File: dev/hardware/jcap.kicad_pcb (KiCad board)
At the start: 2 copper layers, 140 x 87 mm, 74 parts, among them J201 CPU PGMR, J202 GPU PGMR, J203 SPARE GPU HDR, J204 SPARE CPU HDR, J301 DC IN, J502 VGA OUT, J601 CONTROLS, SW201 CPU ~{RES}, SW202 GPU ~{RES}, SW203 DEBUG, SW601 TILT, U101 P8X32A-D40, U201 P8X32A-D40, U302 LF33_TO220, U401 24LC256, U402 24LC256, U601 74HC165, U602 74HC165, Y101 6.5MHz, Y201 6.5MHz

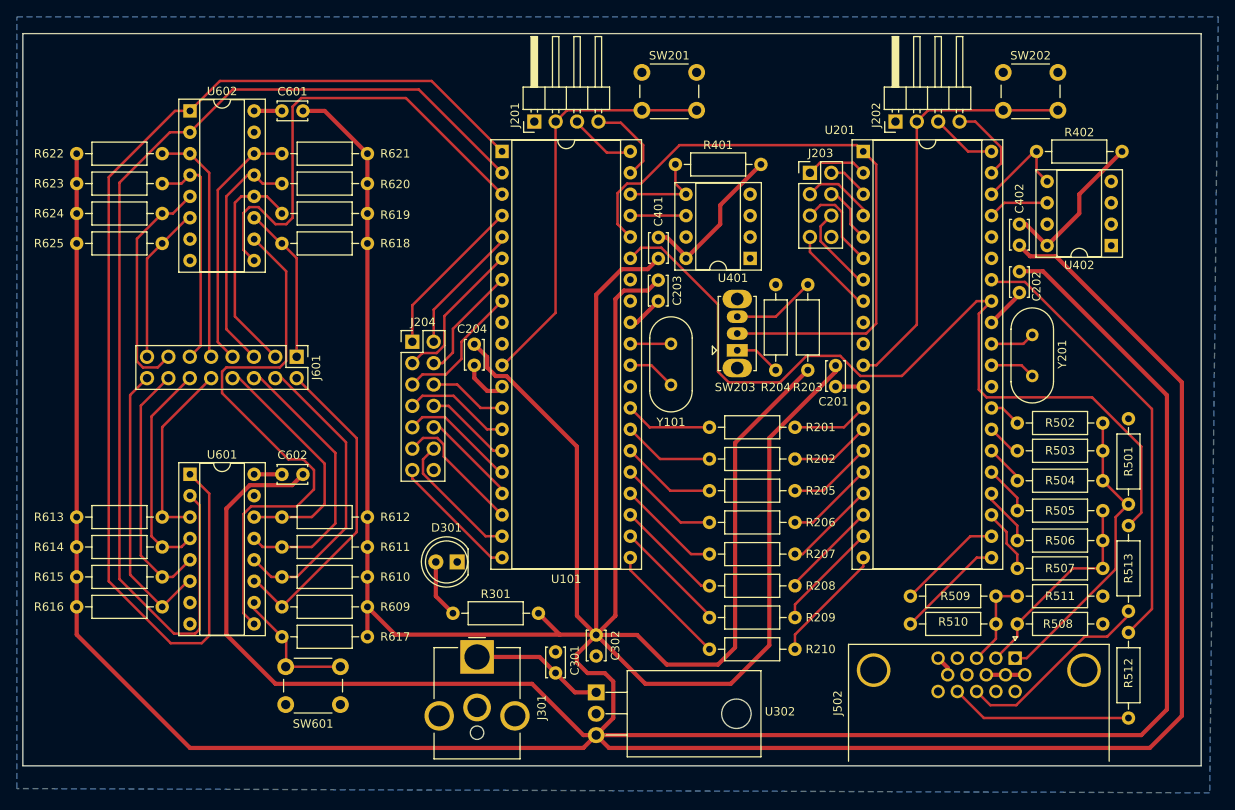
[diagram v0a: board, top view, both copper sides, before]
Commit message: Finalized optimized board layout
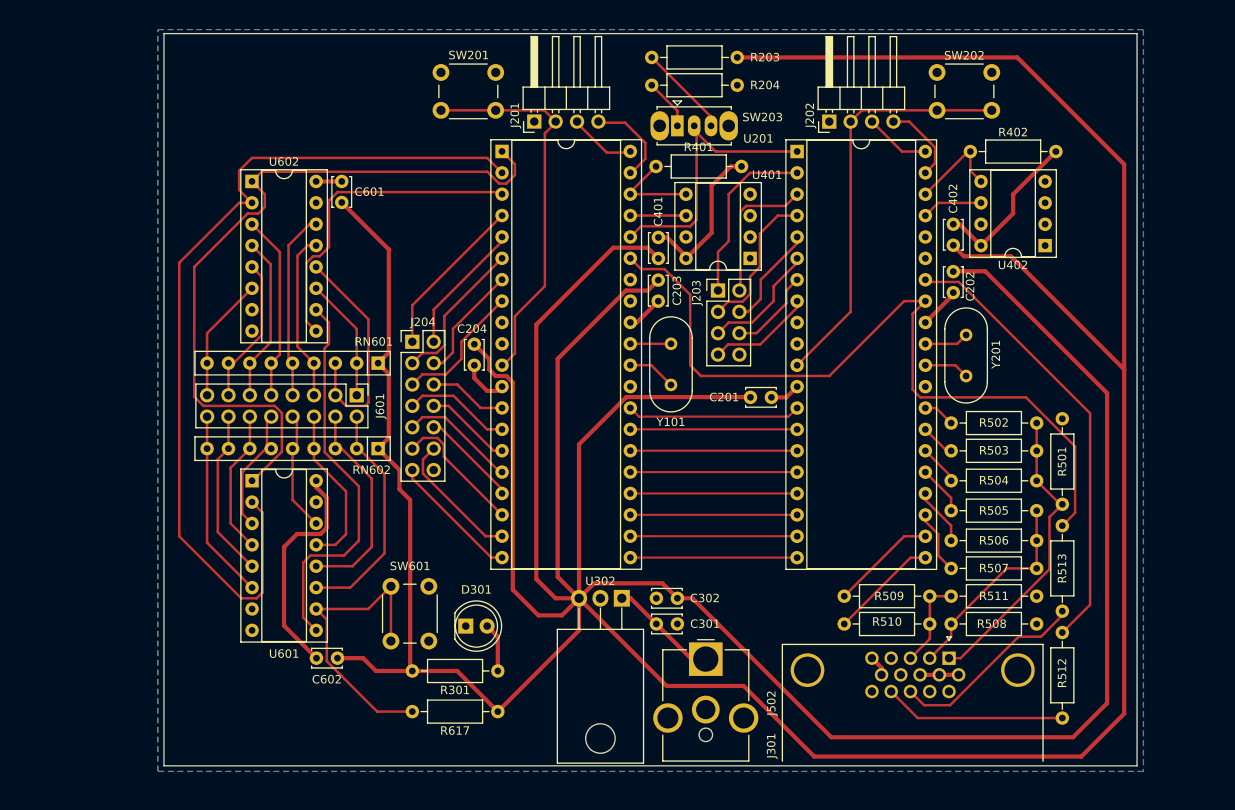
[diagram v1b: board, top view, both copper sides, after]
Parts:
- removed R201, R202, R205, R206, R207, R208, R209, R210: 200, Resistor_THT:R_Axial_DIN0207_L6.3mm_D2.5mm_P10.16mm_Horizontal
- removed R609, R610, R611, R612, R613, R614, R615, R616, R618, R619, R620, R621, R622, R623, R624, R625: 10K, Resistor_THT:R_Axial_DIN0207_L6.3mm_D2.5mm_P10.16mm_Horizontal
- added RN601: 10K, Resistor_THT:R_Array_SIP9, F.Cu at (124.2, 105.2)
- added RN602: 10K, Resistor_THT:R_Array_SIP9, F.Cu at (124.2, 115.3)
- moved R203 32.8 mm to (156.7, 68.8), turned to 0 degrees
- moved SW203 27.6 mm to (159.8, 77.0), turned to 0 degrees
- moved J301 27.2 mm to (163.1, 140.3)
- moved R204 24.1 mm to (166.9, 72.1), turned to 180 degrees
- moved SW201 23.9 mm to (131.7, 70.6)
- moved C602 22.2 mm to (116.9, 140.2)
- moved R617 17.9 mm to (128.3, 146.6)
- moved J203 17.7 mm to (164.6, 96.5)
- moved SW601 17.5 mm to (130.2, 131.7), turned to -90 degrees
- moved R301 16.5 mm to (128.3, 141.7), turned to 0 degrees
- moved C301 14.9 mm to (159.8, 136.1), turned to 180 degrees
- moved U302 11.6 mm to (153.2, 133.1), turned to 180 degrees
- moved U602 11.2 mm to (109.2, 83.6)
- moved C601 11.0 mm to (119.9, 83.6), turned to -90 degrees
- moved C302 9.91 mm to (157.3, 133.1), turned to 0 degrees
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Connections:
- U101 pad 21: /Propellers/CPU_DAT_8 -> /Propellers/GFX_DAT_8
- U101 pad 22: /Propellers/CPU_DAT_7 -> /Propellers/GFX_DAT_7
- U101 pad 23: /Propellers/CPU_DAT_6 -> /Propellers/GFX_DAT_6
- U101 pad 24: /Propellers/CPU_DAT_5 -> /Propellers/GFX_DAT_5
- U101 pad 25: /Propellers/CPU_DAT_4 -> /Propellers/GFX_DAT_4
- U101 pad 26: /Propellers/CPU_DAT_3 -> /Propellers/GFX_DAT_3
- U101 pad 27: /Propellers/CPU_DAT_2 -> /Propellers/GFX_DAT_2
- U101 pad 28: /Propellers/CPU_DAT_1 -> /Propellers/GFX_DAT_1
- U201 pad 13: /Propellers/GPU_DAT_1 -> /Propellers/GFX_DAT_1
- U201 pad 14: /Propellers/GPU_DAT_2 -> /Propellers/GFX_DAT_2
- U201 pad 15: /Propellers/GPU_DAT_3 -> /Propellers/GFX_DAT_3
- U201 pad 16: /Propellers/GPU_DAT_4 -> /Propellers/GFX_DAT_4
- U201 pad 17: /Propellers/GPU_DAT_5 -> /Propellers/GFX_DAT_5
- U201 pad 18: /Propellers/GPU_DAT_6 -> /Propellers/GFX_DAT_6
- U201 pad 19: /Propellers/GPU_DAT_7 -> /Propellers/GFX_DAT_7
- U201 pad 20: /Propellers/GPU_DAT_8 -> /Propellers/GFX_DAT_8
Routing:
- net +3.3V: track 837.9 -> 635.1 mm
- net ~{INPUTS_PL}: track 138.4 -> 87.4 mm
- net /Propellers/DEBUG: track 75.9 -> 33.8 mm
- net INPUTS_CLK: track 130.0 -> 105.6 mm
- net Net-(U601-VCC): track 3.31 -> 26.9 mm
- net /Propellers/GFX_DAT_1: track 0.00 -> 20.7 mm
- net /Input/SHIFT_IN: track 66.9 -> 46.3 mm
- net Net-(U601-DS): track 15.7 -> 35.9 mm
- net /Propellers/GFX_DAT_8: track 0.00 -> 19.8 mm
- net /Propellers/GFX_DAT_7: track 0.00 -> 19.8 mm
- net /Propellers/GFX_DAT_5: track 0.00 -> 19.8 mm
- net /Propellers/GFX_DAT_4: track 0.00 -> 19.8 mm
- net /Propellers/GFX_DAT_2: track 0.00 -> 19.8 mm
- net /Propellers/GFX_DAT_6: track 0.00 -> 19.8 mm
- net /Propellers/GFX_DAT_3: track 0.00 -> 19.8 mm
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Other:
- board size 140 x 87 mm -> 115.6 x 87 mm
